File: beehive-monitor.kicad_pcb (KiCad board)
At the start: 2 copper layers, 90 x 91 mm, 4 parts, among them J1 CONSMA002-L-G, J2 Conn_ARM_JTAG_SWD_10, J3 643270100308, U1 RAK3172

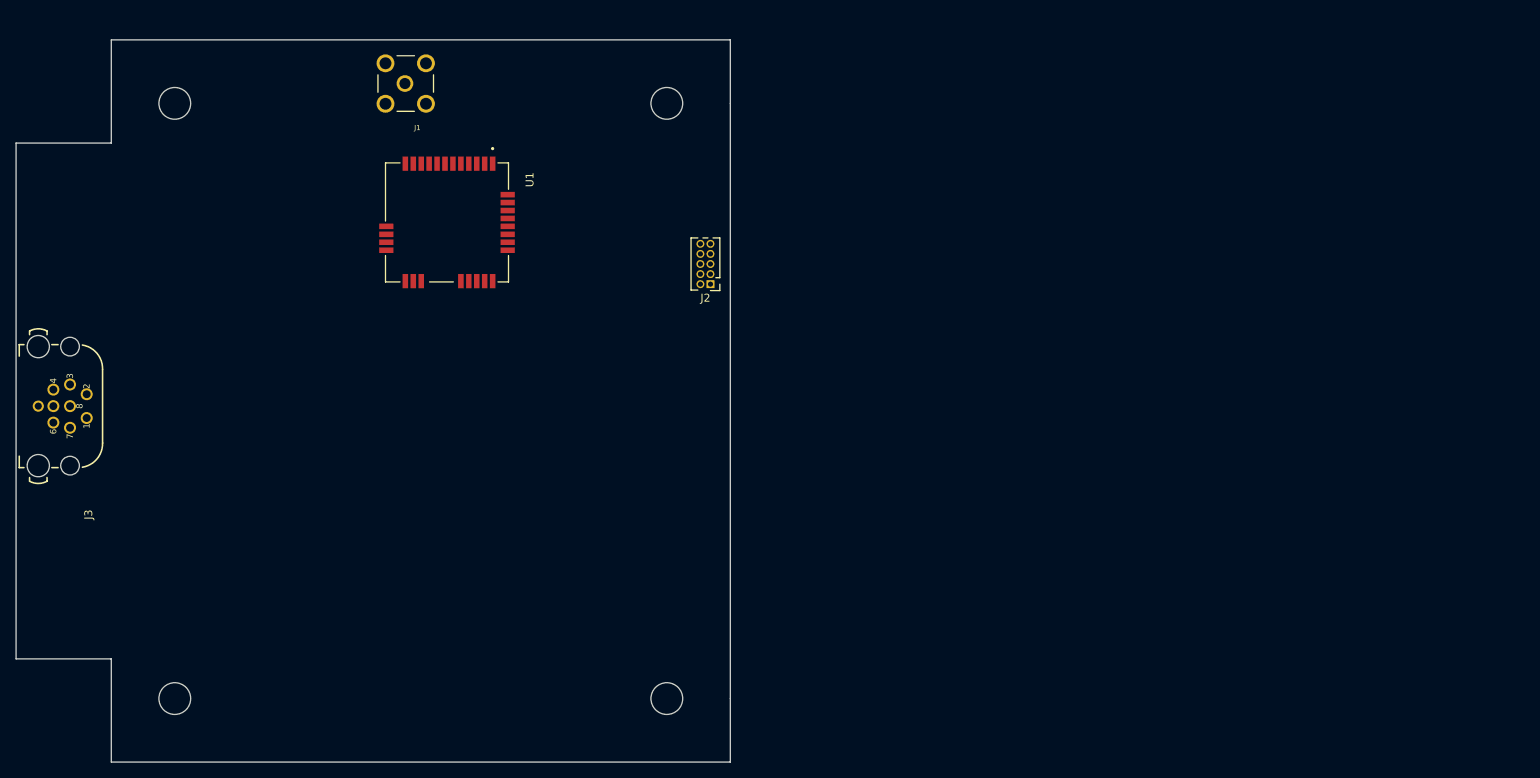
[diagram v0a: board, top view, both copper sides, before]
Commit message: Board
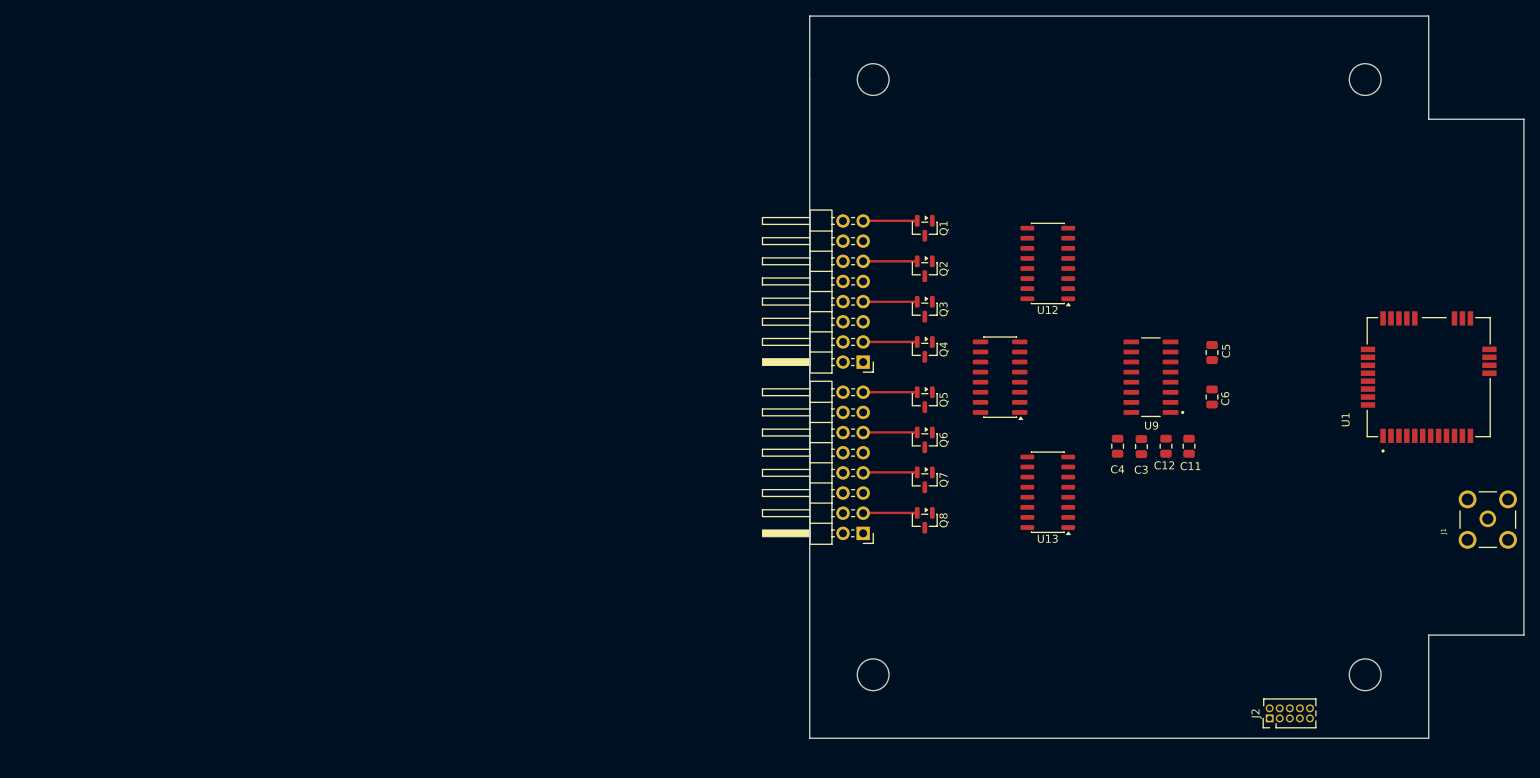
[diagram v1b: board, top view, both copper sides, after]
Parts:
- removed J3: 643270100308, AMQ_FOOTPRINT_LIBRARY:643270100308
- added C11: 10uF, Capacitor_SMD:C_0805_2012Metric, F.Cu at (197.8, 113.2)
- added C12: 100nF, Capacitor_SMD:C_0805_2012Metric, F.Cu at (194.9, 113.2)
- added C3: 10uF, Capacitor_SMD:C_0805_2012Metric, F.Cu at (191.8, 113.2)
- added C4: 100nF, Capacitor_SMD:C_0805_2012Metric, F.Cu at (188.8, 113.2)
- added C5: 0.1uF, Capacitor_SMD:C_0805_2012Metric, F.Cu at (200.7, 101.4)
- added C6: 0.1uF, Capacitor_SMD:C_0805_2012Metric, F.Cu at (200.7, 107.0)
- added J4: Conn_02x08_Odd_Even, Connector_PinHeader_2.54mm:PinHeader_2x08_P2.54mm_Horizontal, F.Cu at (156.7, 124.2)
- added J5: Conn_02x08_Odd_Even, Connector_PinHeader_2.54mm:PinHeader_2x08_P2.54mm_Horizontal, F.Cu at (156.7, 102.6)
- added Q1: Q_PMOS_GSD, Package_TO_SOT_SMD:SOT-23, F.Cu at (164.5, 85.7)
- added Q2: Q_PMOS_GSD, Package_TO_SOT_SMD:SOT-23, F.Cu at (164.5, 90.8)
- added Q3: Q_PMOS_GSD, Package_TO_SOT_SMD:SOT-23, F.Cu at (164.5, 95.9)
- added Q4: Q_PMOS_GSD, Package_TO_SOT_SMD:SOT-23, F.Cu at (164.5, 101.0)
- added Q5: Q_PMOS_GSD, Package_TO_SOT_SMD:SOT-23, F.Cu at (164.5, 107.3)
- added Q6: Q_PMOS_GSD, Package_TO_SOT_SMD:SOT-23, F.Cu at (164.5, 112.4)
- added Q7: Q_PMOS_GSD, Package_TO_SOT_SMD:SOT-23, F.Cu at (164.5, 117.4)
- added Q8: Q_PMOS_GSD, Package_TO_SOT_SMD:SOT-23, F.Cu at (164.5, 122.5)
- added U10: 74HC138, Package_SO:SOIC-16_3.9x9.9mm_P1.27mm, F.Cu at (174.0, 104.5)
- added U12: 74HC4051, Package_SO:SO-16_3.9x9.9mm_P1.27mm, F.Cu at (180.0, 90.2)
- added U13: 74HC4051, Package_SO:SO-16_3.9x9.9mm_P1.27mm, F.Cu at (180.0, 119.0)
- added U9: NAU7802SGI, AMQ_FOOTPRINT_LIBRARY:SOIC127P600X175-16N, F.Cu at (193.0, 104.5)
- moved J1 147.0 mm to (235.4, 122.5), turned to 90 degrees
- moved U1 125.2 mm to (228.0, 104.5), turned to 90 degrees
- moved J2 89.2 mm to (208.0, 147.5), turned to 90 degrees
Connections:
- U1 pad 10: unconnected-(U1-PA11/I2C_SDA-Pad10) -> NAU7802_SDIO
- U1 pad 29: unconnected-(U1-PA0-Pad29) -> LC_SELECTOR_00
- U1 pad 3: unconnected-(U1-PA15/PIN_A4-Pad3) -> LC_SELECTOR_02
- U1 pad 6: unconnected-(U1-PA1-Pad6) -> LC_SELECTOR_01
- U1 pad 9: unconnected-(U1-PA12/I2C_SCL-Pad9) -> NAU7802_SCK
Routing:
- net LC_02_EXC_POS: track 0.00 -> 6.83 mm
- net LC_01_EXC_POS: track 0.00 -> 6.83 mm
- net LC_08_EXC_POS: track 0.00 -> 6.82 mm
- net LC_06_EXC_POS: track 0.00 -> 6.82 mm
- net LC_03_EXC_POS: track 0.00 -> 6.82 mm
- net LC_05_EXC_POS: track 0.00 -> 6.81 mm
- net LC_07_EXC_POS: track 0.00 -> 6.81 mm
- net LC_04_EXC_POS: track 0.00 -> 6.81 mm
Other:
- outline, holes or cut-outs redrawn
- copper layers 2 -> 4
- board text added: "(150,150)"
- board text added: "(150,59)"
- board text added: "(228,150)"
- board text added: "(240,137)"
